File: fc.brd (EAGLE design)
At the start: 55 x 40 mm, 72 parts, among them IC1 BN055, J1 USBC, U1 LMZ21700, U2 ATMEGA2560-16AU100A-M, U4 FT230XQ, Y1 16MHz, Y2 32.768kHz

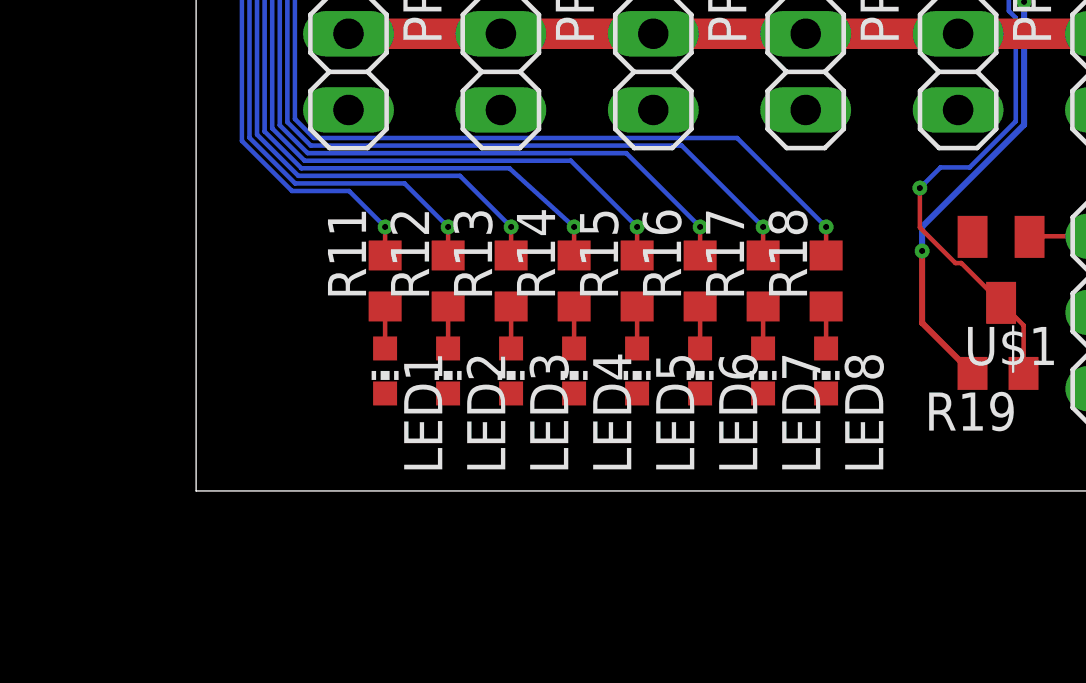
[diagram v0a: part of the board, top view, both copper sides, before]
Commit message: led placement on grid
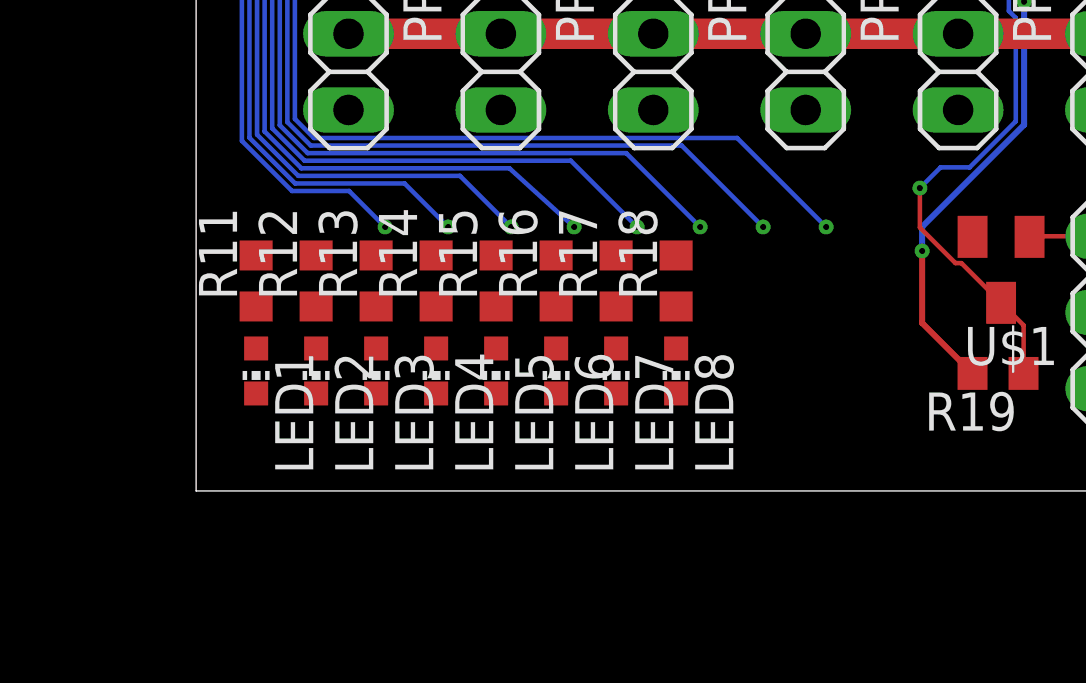
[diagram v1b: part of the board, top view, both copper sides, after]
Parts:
- moved LED8 5.00 mm to (16.0, 4.00)
- moved R18 5.00 mm to (16.0, 7.00)
- moved LED7 4.90 mm to (14.0, 4.00)
- moved R17 4.90 mm to (14.0, 7.00)
- moved LED6 4.80 mm to (12.0, 4.00)
- moved R16 4.80 mm to (12.0, 7.00)
- moved LED5 4.70 mm to (10.0, 4.00)
- moved R15 4.70 mm to (10.0, 7.00)
- moved LED4 4.60 mm to (8.00, 4.00)
- moved R14 4.60 mm to (8.00, 7.00)
- moved LED3 4.50 mm to (6.00, 4.00)
- moved R13 4.50 mm to (6.00, 7.00)
- moved LED2 4.40 mm to (4.00, 4.00)
- moved R12 4.40 mm to (4.00, 7.00)
- moved LED1 4.30 mm to (2.00, 4.00)
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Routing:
- net N$31: track 1.40 -> 0.00 mm
- net N$29: track 1.40 -> 0.00 mm
- net N$27: track 1.40 -> 0.00 mm
- net N$24: track 1.40 -> 0.00 mm
- net N$22: track 1.40 -> 0.00 mm
- net N$20: track 1.40 -> 0.00 mm
- net N$18: track 1.40 -> 0.00 mm
- net N$15: track 1.40 -> 0.00 mm
- net LED1: track 38.6 -> 37.7 mm
- net LED7: track 46.2 -> 45.3 mm
- net LED6: track 45.0 -> 44.1 mm
- net LED5: track 43.7 -> 42.8 mm
- net LED4: track 42.4 -> 41.5 mm
- net LED3: track 41.1 -> 40.2 mm
- net LED2: track 39.9 -> 39.0 mm
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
